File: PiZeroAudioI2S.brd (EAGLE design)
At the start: 65.1 x 30.2 mm, 68 parts, among them CON1 RPI-Header, J1 GROVE, J2 2X2HEADER, J3 2X1-LOCKING, J4 GROVE, J5 4X1-LOCKING, Q1 DMG2305UX, U1 TXB0104PWR, U2 LSM6DS33, U3 PCM5101A, U5 TXS0102, U6 TPA3144D2PWPR

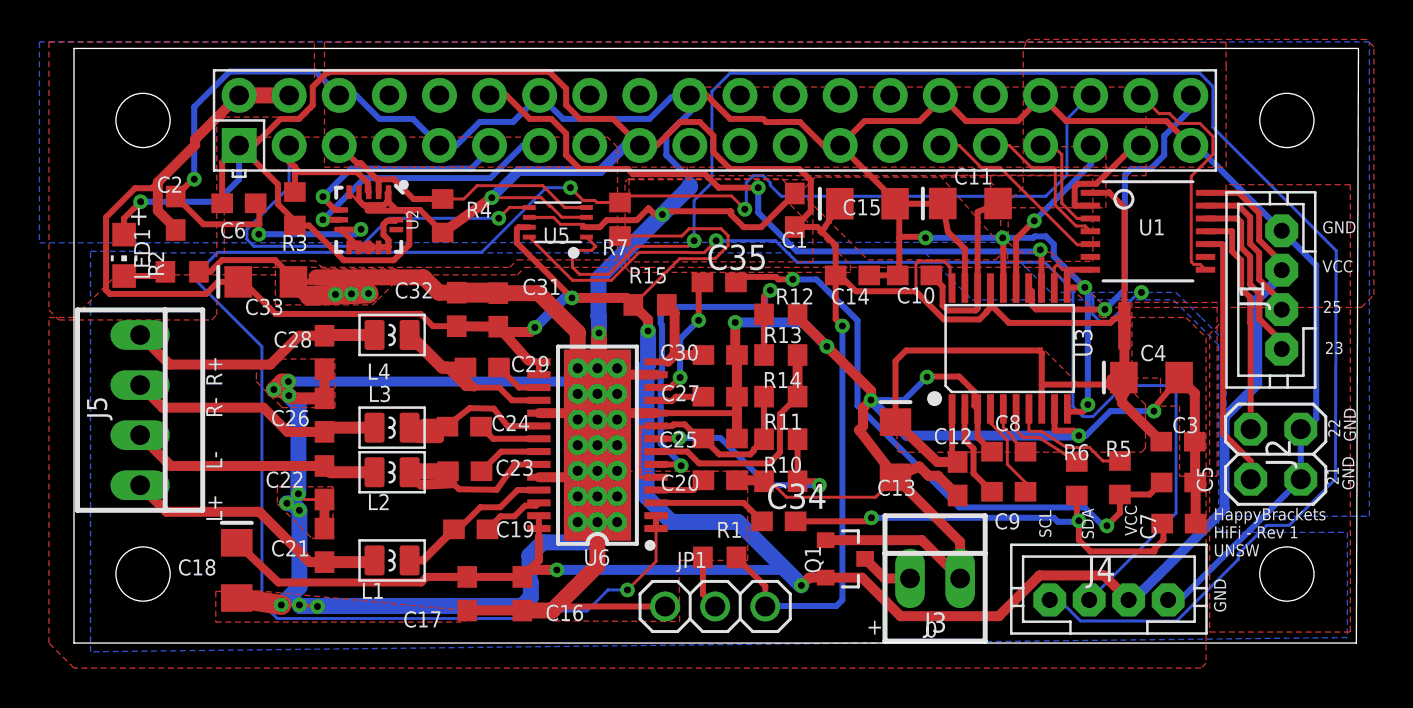
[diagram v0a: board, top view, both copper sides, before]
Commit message: Adjusted Layout
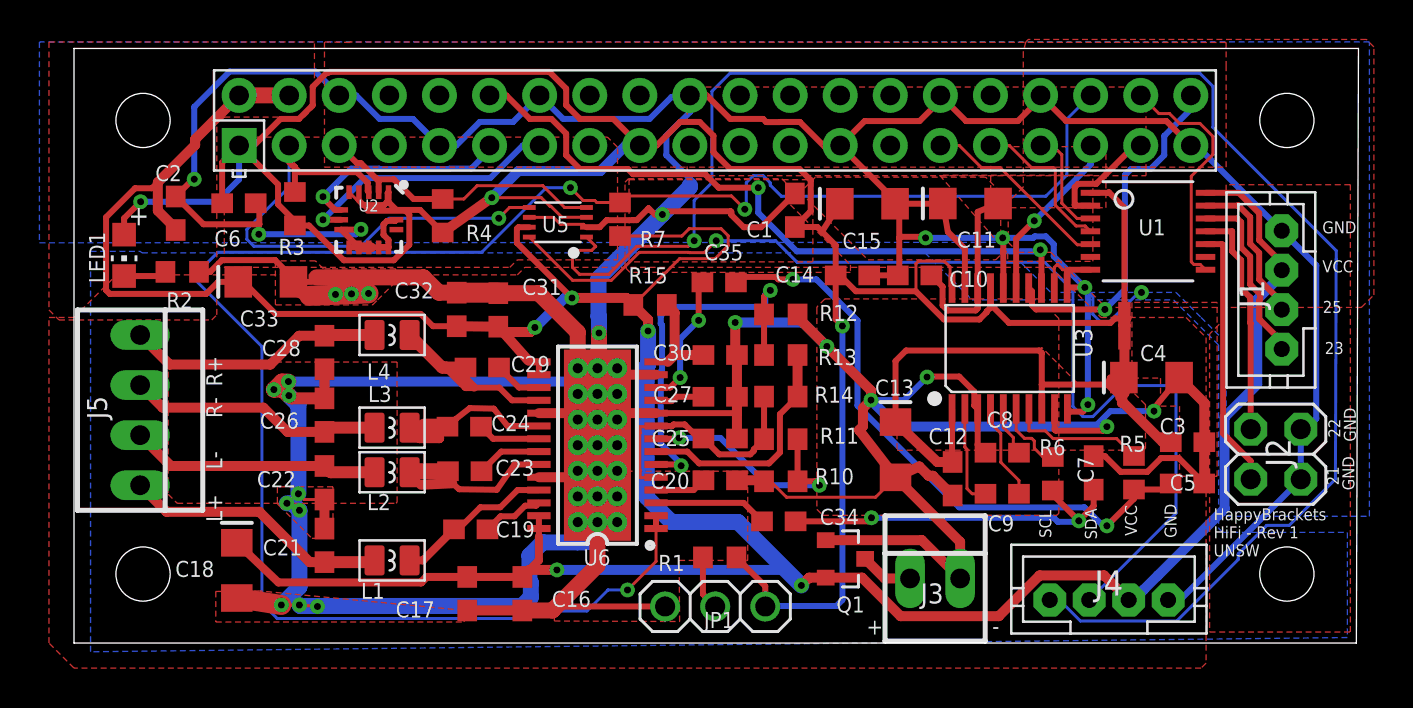
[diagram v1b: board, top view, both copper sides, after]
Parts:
- moved C7 5.03 mm to (-27.0, 9.90), turned to 90 degrees
- moved R6 1.25 mm to (-29.1, 9.86)
- moved R5 0.76 mm to (-25.0, 9.91)
- moved C3 0.48 mm to (-22.3, 11.5)
- moved C5 0.46 mm to (-22.3, 9.36)
- moved C9 0.35 mm to (-31.7, 8.84)
- moved C8 0.33 mm to (-31.7, 10.9)
- moved C12 0.25 mm to (-34.2, 9.60)
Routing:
- net AGND: track 269.2 -> 276.1 mm
- net AUDIO-LEFT: track 22.5 -> 18.5 mm
- net N$11: track 4.68 -> 3.71 mm
- net N$1: track 6.26 -> 6.96 mm
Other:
- board text added: "-"
- board text removed: "0"

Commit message: Build Revision 1
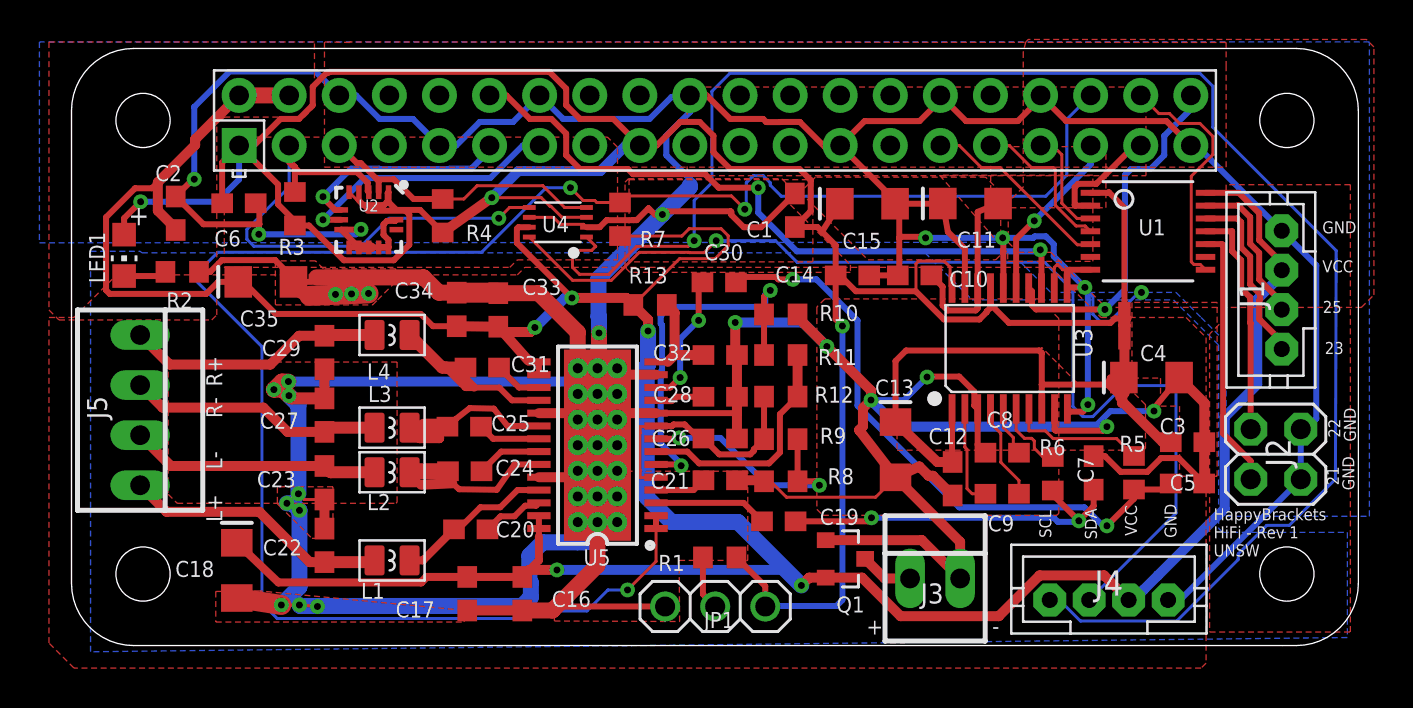
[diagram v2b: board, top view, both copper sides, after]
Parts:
- removed R14: 33K, adafruit:R0603
- removed R15: 10R, adafruit:R0603
- removed U6: TPA3144D2PWPR, HappyBrackets:HTSSOP28
- added R8: 39K, adafruit:R0603
- added R9: 56K, adafruit:R0603
- added U4: TXS0102, adafruit:VFSOP-8
- C19: value 220nF -> 1uF
- C20, C25: value 1uF -> 220nF
- C21, C26, C28: value 1nF -> 1uF
- C23, C29: value 220nF -> 1nF
- C27: value 1uF -> 1nF
- C31: value 1nF -> 220nF
- C32: value 0.1uF -> 1uF
- C33: value 100uF -> 1nF; device HappyBrackets:EIA3216 -> rcl:C0603
- C34: value 1uF -> 0.1uF
- C35: value 1uF -> 100uF; device rcl:C0603 -> HappyBrackets:EIA3216
- R10: value 39K -> 33K
- R11: value 56K -> 33K
- R13: value 33K -> 10R
- R5, R6: value 470 -> 80K
- U5: value TXS0102 -> TPA3144D2PWPR; device adafruit:VFSOP-8 -> HappyBrackets:HTSSOP28
- moved C35 23.0 mm to (-69.0, 19.6), turned to 180 degrees
- moved C21 20.3 mm to (-46.0, 9.53), turned to 0 degrees
- moved C28 20.2 mm to (-46.0, 13.8), turned to 0 degrees
- moved C26 20.1 mm to (-46.0, 11.6), turned to 0 degrees
- moved C27 20.1 mm to (-66.0, 12.8), turned to 90 degrees
- moved C34 19.5 mm to (-59.3, 18.2), turned to 90 degrees
- moved C19 15.6 mm to (-43.0, 7.44)
- moved C32 13.6 mm to (-46.0, 15.9), turned to 0 degrees
- moved C25 13.0 mm to (-59.0, 12.2)
- moved C20 12.9 mm to (-58.6, 7.04)
- moved C33 11.9 mm to (-57.2, 18.2), turned to 90 degrees
- moved U5 11.5 mm to (-52.2, 11.3)
- moved R10 8.46 mm to (-42.9, 17.9), turned to 0 degrees
- moved C29 8.04 mm to (-66.0, 16.0), turned to 90 degrees
- moved C23 7.14 mm to (-66.0, 9.40), turned to 90 degrees
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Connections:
- net +3V3: now also U4.P$3; no longer U5.P$3
- net +5V: now also C33.1, C34.1, C35.+, R13.2, U4.P$7, U5.15, U5.16, U5.27, U5.28; no longer C31.1, C32.1, C33.+, R15.2, U5.P$7, U6.15, U6.16, U6.27, U6.28
- net /MUTE: now also U5.1, U5.2; no longer U6.1, U6.2
- net AGND: now also C22.2, C23.1, C28.2, C29.1, C33.2, C34.2, C35.-, R8.2, U5.10, U5.13, U5.19, U5.24, U5.GND@10, U5.GND@11, U5.GND@12, U5.GND@13, U5.GND@14, U5.GND@15, U5.GND@16, U5.GND@17, U5.GND@18, U5.GND@19, U5.GND@20, U5.GND@21, U5.GND@22, U5.GND@23, U5.GND@24, U5.GND@25, U5.GND@26, U5.GND@27, U5.GND@28, U5.GND@29, U5.GND@30, U5.GND@PAD; no longer C20.2, C22.1, C25.2, C28.1, C30.2, C31.2, C33.-, R12.2, U6.10, U6.13, U6.19, U6.24, U6.GND@10, U6.GND@11, U6.GND@12, U6.GND@13, U6.GND@14, U6.GND@15, U6.GND@16, U6.GND@17, U6.GND@18, U6.GND@19, U6.GND@20, U6.GND@21, U6.GND@22, U6.GND@23, U6.GND@24, U6.GND@25, U6.GND@26, U6.GND@27, U6.GND@28, U6.GND@29, U6.GND@30, U6.GND@PAD
- net AUDIO-LEFT: now also C19.2; no longer C34.2
- net AUDIO-RIGHT: now also C30.2; no longer C35.2
- net GND: now also U4.P$2, U4.P$6; no longer U5.P$2, U5.P$6
- net L+: now also C22.1; no longer C21.1
- net L-: now also C23.2; no longer C22.2
- net N$10: now also C31.2, U5.17; no longer C29.2, U6.17
- net N$13: now also C25.2, U5.21; no longer C24.2, U6.21
- net N$14: now also C19.1, U5.3; no longer C34.1, U6.3
- net N$15: now also C30.1, U5.12; no longer C35.1, U6.12
- net N$16: now also C24.2, U5.22; no longer C23.2, U6.22
- net N$17: now also C20.2, U5.26; no longer C19.2, U6.26
- net N$18: now also C20.1, U5.25; no longer C19.1, U6.25
- net N$19: now also C24.1, U5.23; no longer C23.1, U6.23
- net N$20: now also C25.1, U5.20; no longer C24.1, U6.20
- net N$21: now also C31.1, U5.18; no longer C29.1, U6.18
- net N$23: now also R10.1, R11.2, U5.6; no longer R12.1, R13.2, U6.6
- net N$24: now also R11.1, R12.2, U5.7; no longer R13.1, R14.2, U6.7
- net N$25: now also R8.1, R9.2, U5.8; no longer R10.1, R11.2, U6.8
- net N$26: now also C26.1, R12.1, R9.1, U5.5, U5.9; no longer C25.1, R11.1, R14.1, U6.5, U6.9
- net N$7: now also C21.1, U5.4; no longer C20.1, U6.4
- net N$8: now also C28.1, U5.11; no longer C27.1, U6.11
- net N$9: now also C32.1, R13.1, U5.14; no longer C30.1, R15.1, U6.14
- net R+: now also C29.2; no longer C28.2
- net R-: now also C27.1; no longer C26.1
- net SCL: now also U4.P$4; no longer U5.P$4
- net SCL-OUT: now also U4.P$1; no longer U5.P$1
- net SDA: now also U4.P$5; no longer U5.P$5
- net SDA-OUT: now also U4.P$8; no longer U5.P$8
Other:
- board size 65.1 x 30.2 mm -> 65.3 x 30.3 mm
